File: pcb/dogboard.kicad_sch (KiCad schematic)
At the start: 32 parts, among them J1 USB-C / USB2.0, SW2 BOOT, U1 RP2040, U3 4MB Flash, Y1 12 MHz

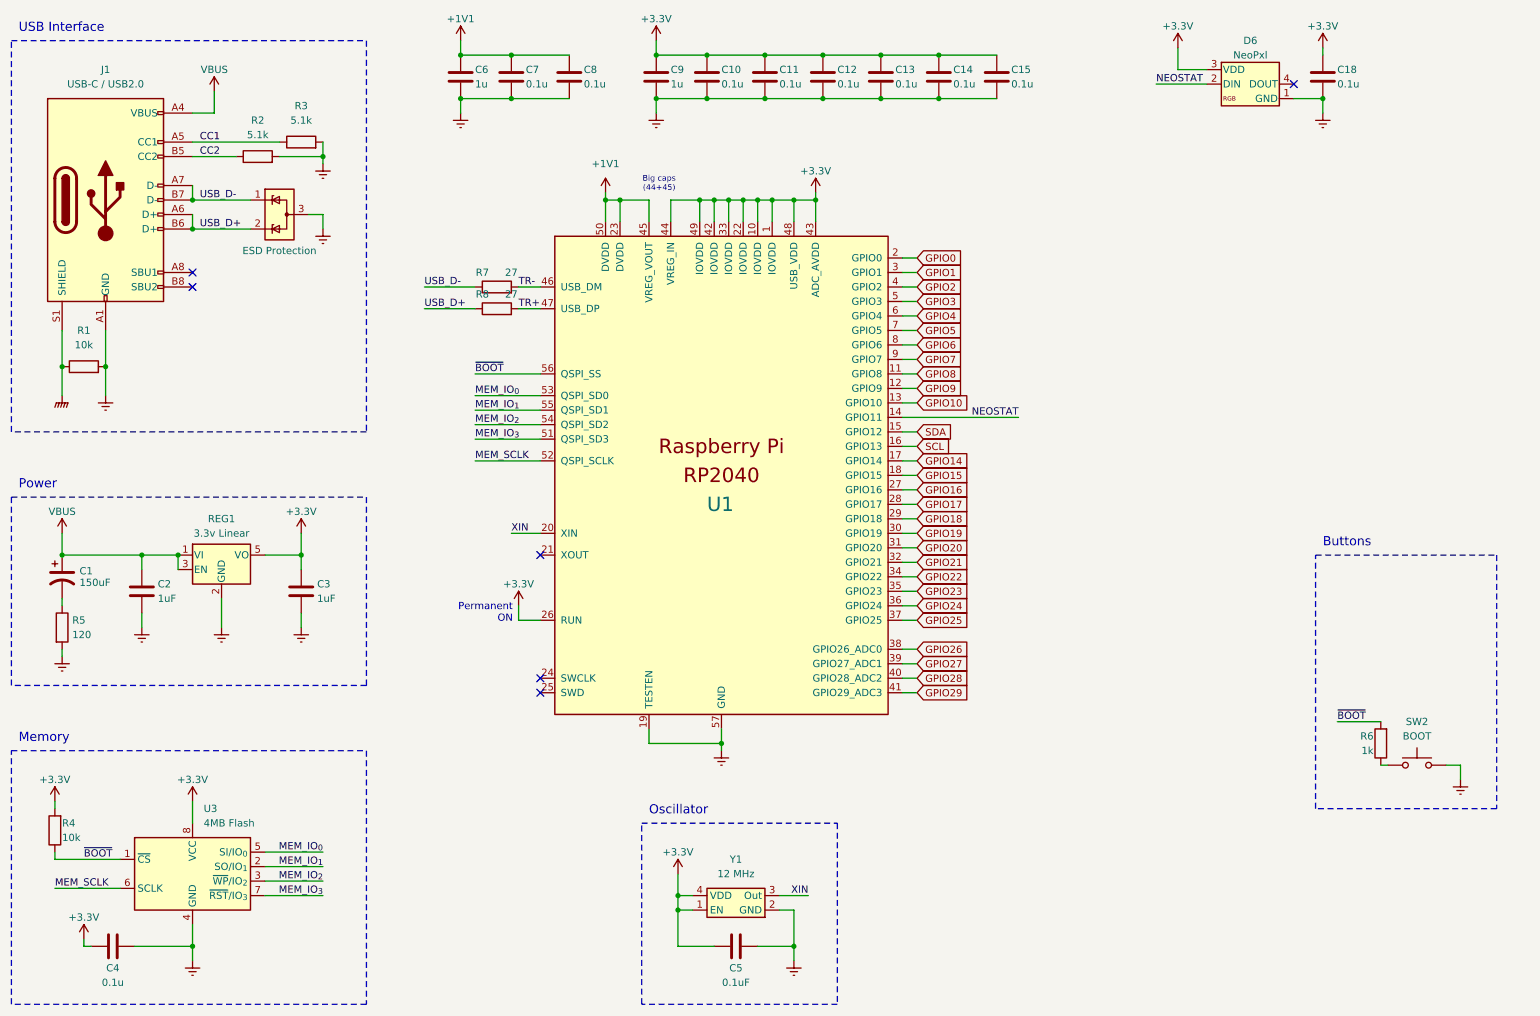
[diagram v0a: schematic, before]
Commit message: PBC rev 2 beta-1
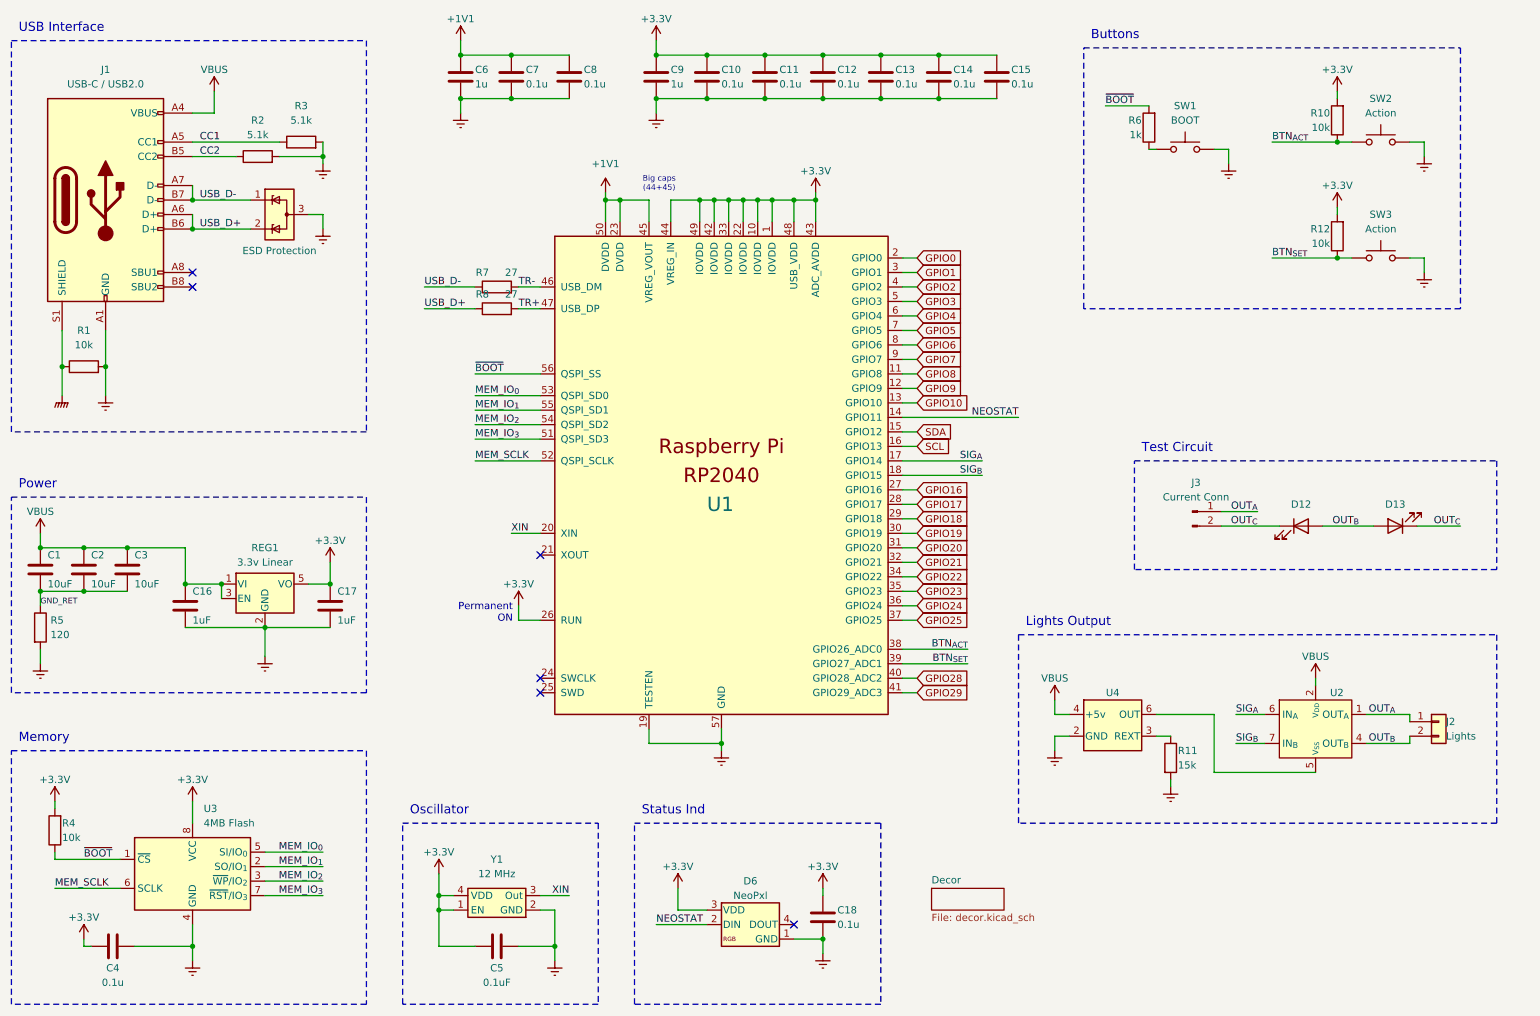
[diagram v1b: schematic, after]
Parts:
- removed C1: 150uF, _custom:CAP_Tantalum_2312, symbol _custom:CAP_Tantalum
- added C1: 10uF, _custom:CAP_1206_NoKeepout, symbol _custom:CAP_Standard
- added C16, C17: 1uF, _custom:CAP_0805_HandSolder, symbol _custom:CAP_Standard
- added D12, D13: MP-LED, _custom:LED_MP-Cathode_1113, symbol _custom:LED_Standard
- added J2: Lights, _custom:conn_1x02_JST_PH_P2.00mm_THT_Horizontal, symbol _custom:Conn_1x02
- added J3: Current Conn, Connector_PinHeader_2.54mm:PinHeader_1x02_P2.54mm_Vertical, symbol Connector:Conn_01x02_Pin
- added R10, R12: 10k, _custom:R_0805_HandSolder, symbol _custom:Resistor_Standard
- added R11: 15k, _custom:R_0805_HandSolder, symbol _custom:Resistor_Standard
- added SW2, SW3: Action, _custom:button_SMD_PTS810, symbol _custom:SW_Button_Push
- added U2: L9110H, _custom:GenericIC_TH-DIP-8, symbol _custom:L9110H_H-Bridge
- added U4: BCR430, _custom:BCR430_CC_LED_Driver, symbol _custom:BCR430_CC_LED_Driver
- C2, C3: value 1uF -> 10uF; footprint _custom:CAP_0805_HandSolder -> _custom:CAP_1206_NoKeepout
- renumbered SW2 to SW1
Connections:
- net +3.3V: now also C17.1, R10.2, R12.2; no longer C3.2
- net GNDREF: now also C16.2, C17.2, R11.2, SW2.2, SW3.2, U4.2 (GND); no longer C2.1, C3.1
- net VBUS: now also C2.1, C3.1, C1.1, C16.1, U2.2 (V_{DD}), U2.3 (V_{DD}), U4.4 (+5v); no longer C2.2
- net GND_RET: now reaches R5.1
- net GND_RET: now also C2.2, C3.2, C1.2
- net GPIO14 renamed SIG_{A}
- net SIG_{A}: now also U2.6 (IN_{A})
- net GPIO15 renamed SIG_{B}
- net SIG_{B}: now also U2.7 (IN_{B})
- net GPIO26 renamed BTN_{ACT}
- net BTN_{ACT}: now also R10.1, SW2.1
- net GPIO27 renamed BTN_{SET}
- net BTN_{SET}: now also R12.1, SW3.1
- new net: R11.1, U4.3 (REXT)
- new net OUT_{A}: J2.1 (Pin_1), J3.1 (Pin_1), U2.1 (OUT_{A})
- new net OUT_{B}: D12.2 (A), D13.2 (A), J2.2 (Pin_2), U2.4 (OUT_{B})
- new net OUT_{C}: D12.1 (K), D13.1 (K), J3.2 (Pin_2)
- new net V_{SS}: U2.5 (V_{SS}), U2.8 (V_{SS}), U4.6 (OUT)
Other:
- added sheet Decor (decor.kicad_sch)
- note added: "Lights Output"
- note added: "Status Ind"
- note added: "Test Circuit"
- moved on the sheet: C18, C5, D6, R5, R6, REG1, SW1, Y1

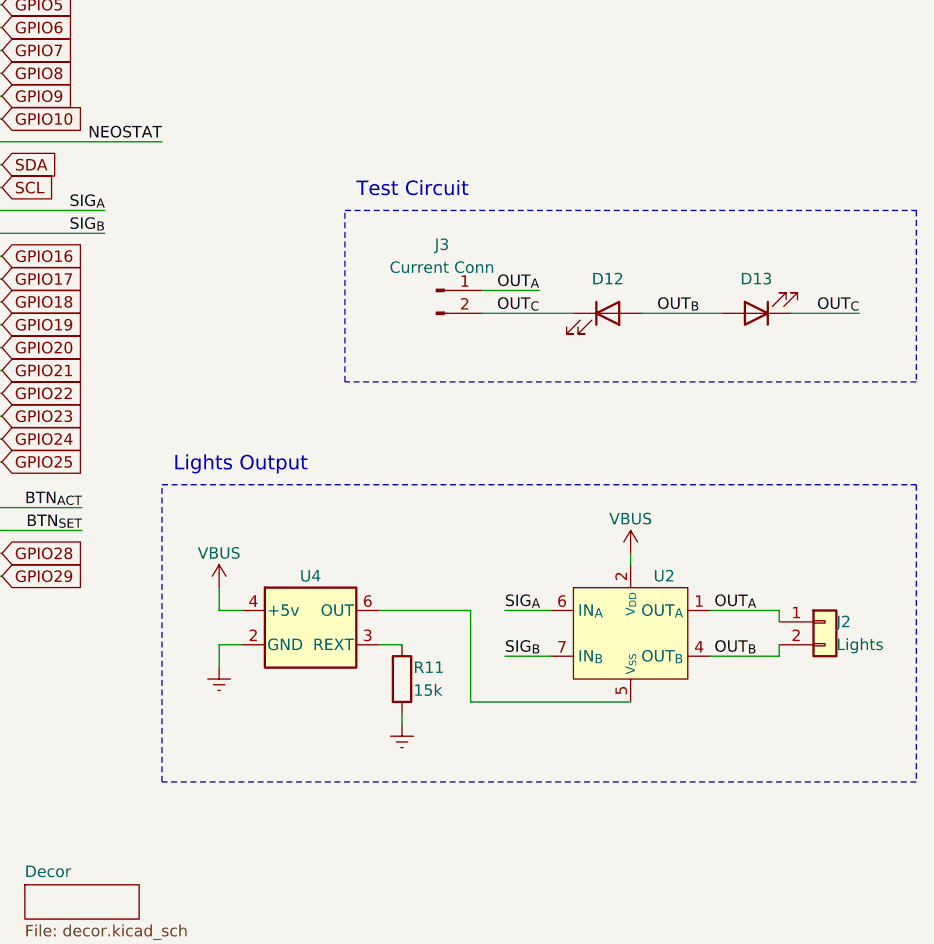
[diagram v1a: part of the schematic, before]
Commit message: PCB rev 2 beta-2
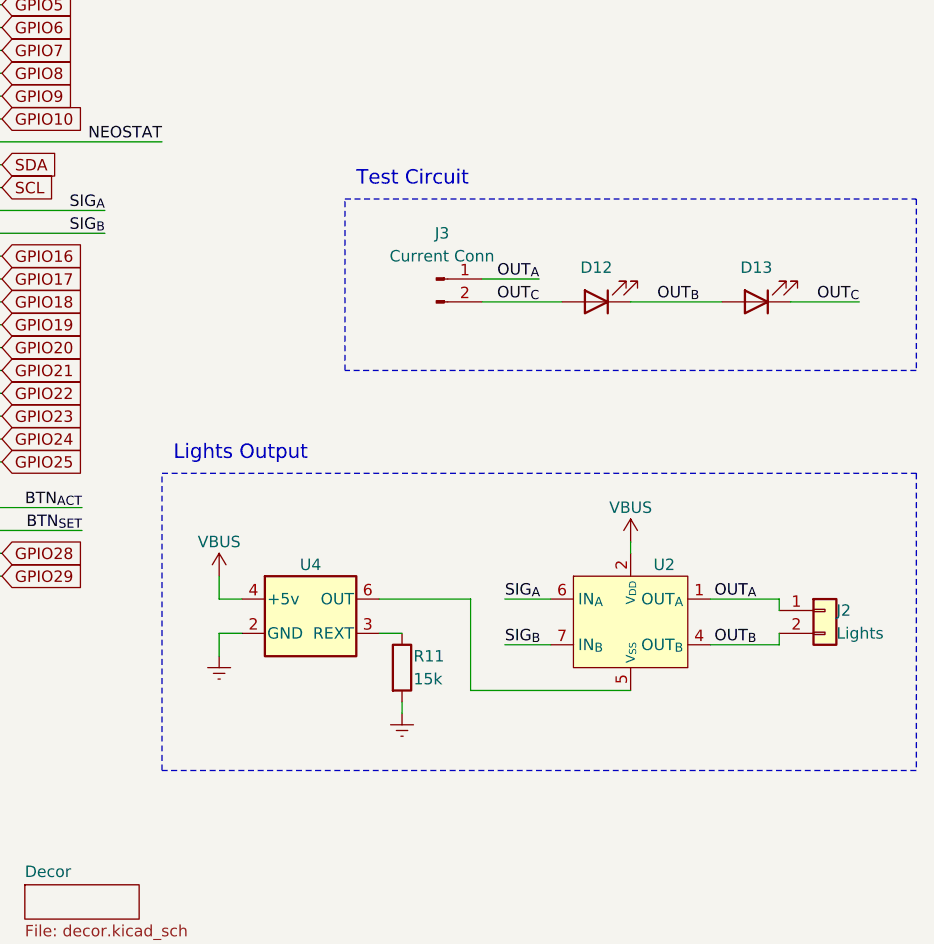
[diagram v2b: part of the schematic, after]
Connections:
- net OUT_{B}: now also D12.1 (K); no longer D12.2 (A)
- net OUT_{C}: now also D12.2 (A); no longer D12.1 (K)
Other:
- moved on the sheet: D12, D13, J2, J3, R11, U2, U4

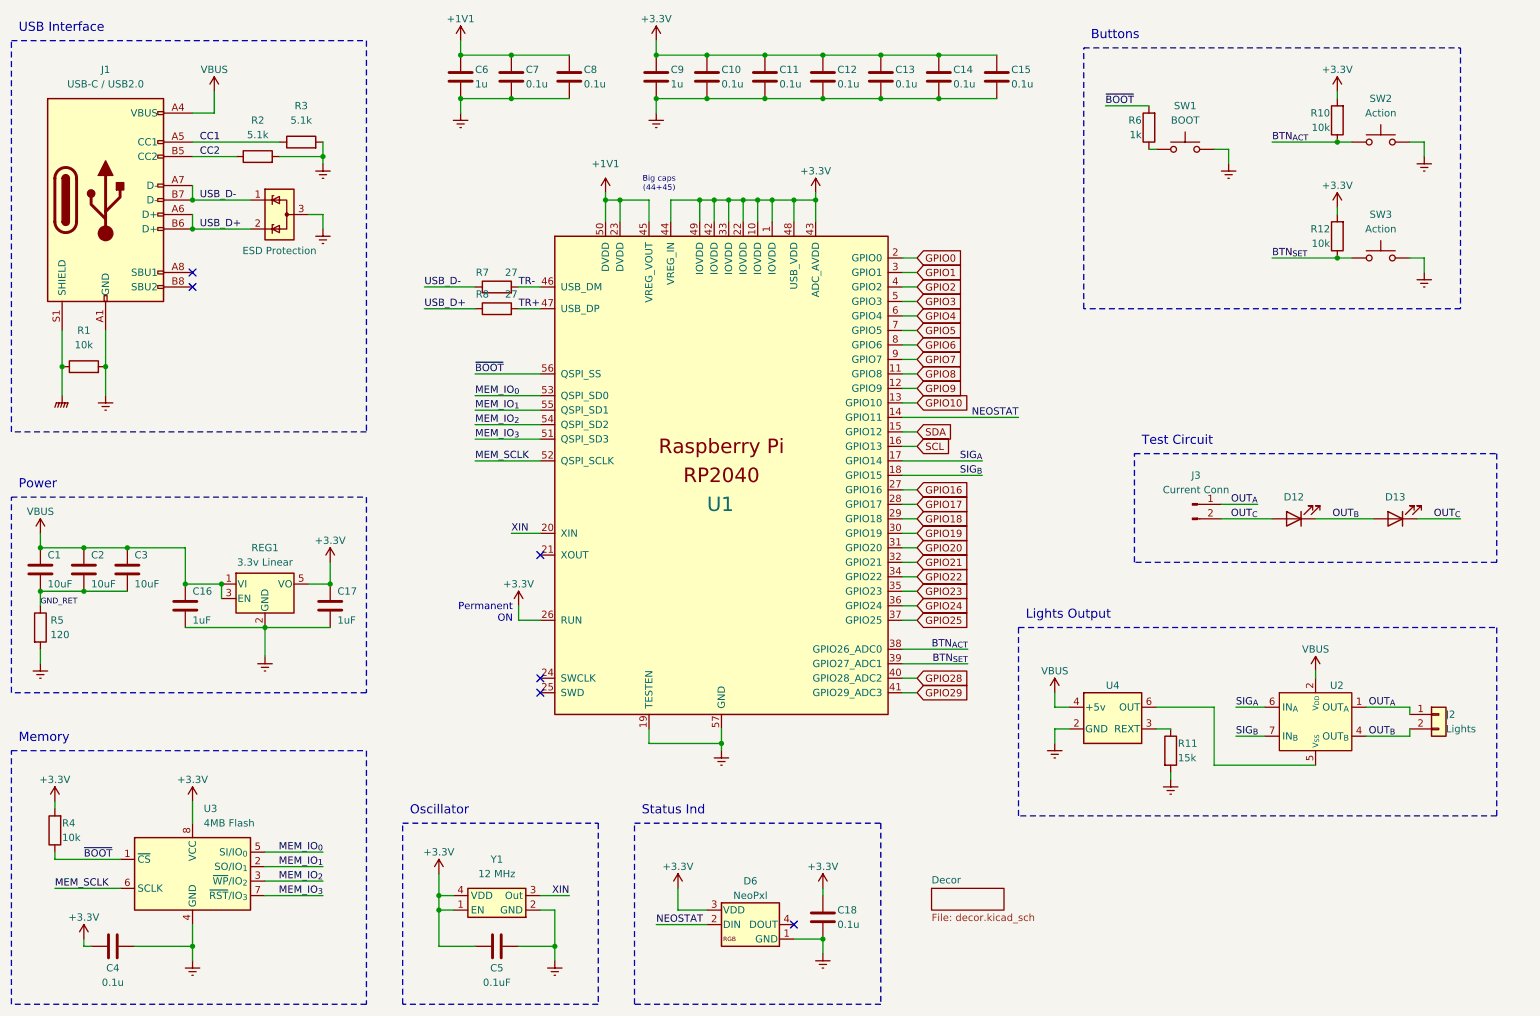
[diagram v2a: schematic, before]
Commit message: dogboard-2b3
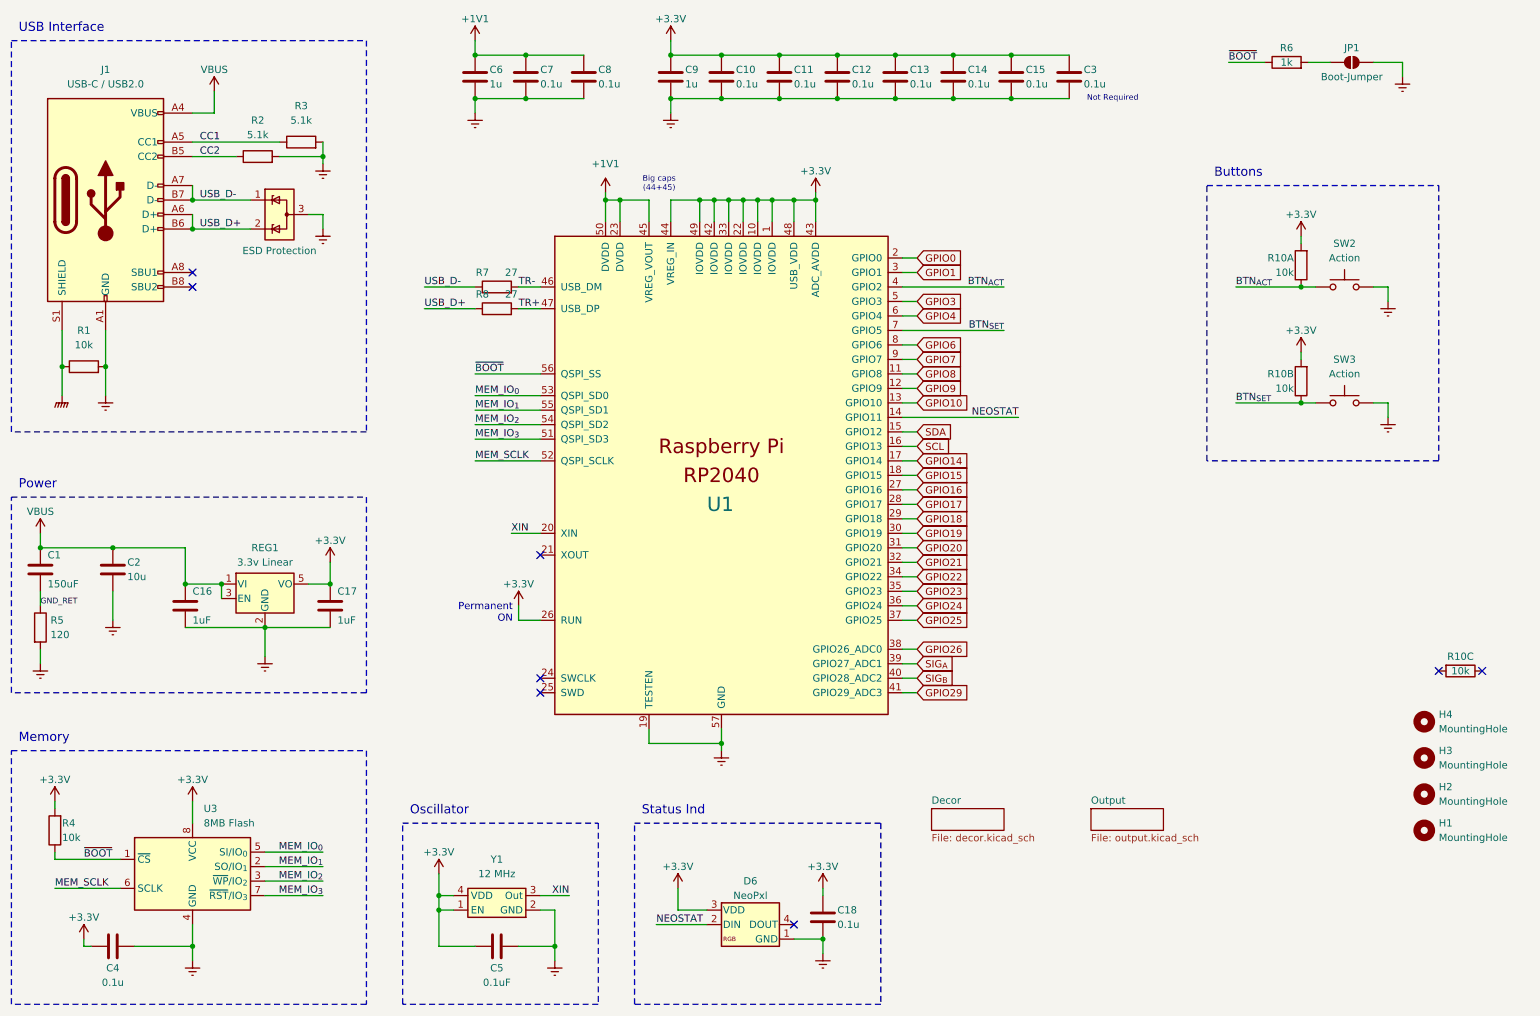
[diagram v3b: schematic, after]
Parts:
- removed D12, D13: MP-LED, _custom:LED_MP-Cathode_1113, symbol _custom:LED_Standard
- removed J2: Lights, _custom:conn_1x02_JST_PH_P2.00mm_THT_Horizontal, symbol _custom:Conn_1x02
- removed J3: Current Conn, Connector_PinHeader_2.54mm:PinHeader_1x02_P2.54mm_Vertical, symbol Connector:Conn_01x02_Pin
- removed R10, R12: 10k, _custom:R_0805_HandSolder, symbol _custom:Resistor_Standard
- removed R11: 15k, _custom:R_0805_HandSolder, symbol _custom:Resistor_Standard
- removed SW1: BOOT, _custom:button_metal_smd, symbol _custom:SW_Button_Push
- removed U2: L9110H, _custom:GenericIC_TH-DIP-8, symbol _custom:L9110H_H-Bridge
- removed U4: BCR430, _custom:BCR430_CC_LED_Driver, symbol _custom:BCR430_CC_LED_Driver
- added H1, H2, H3, H4: MountingHole, _custom:MountingHole_M2.5, symbol _custom:MountingHole
- added JP1: Boot-Jumper, _custom:Jumper_Open_SMD_3.5mm, symbol _custom:Jumper_Open
- added R10: 10k, _custom:R_Array_4x1206_Convex, symbol _custom:Resistor_Array_4x
- C1: value 10uF -> 150uF; footprint _custom:CAP_1206_NoKeepout -> _custom:CAP_Tantalum_2312
- C2: value 10uF -> 10u
- C3: value 10uF -> 0.1u; footprint _custom:CAP_1206_NoKeepout -> _custom:CAP_0402_HandSolder
- R4, R6: footprint _custom:R_0805_HandSolder -> _custom:R_0603_HandSolder
- U3: value 4MB Flash -> 8MB Flash
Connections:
- net GPIO2 is gone; now on net BTN_{ACT}: U1.4 (GPIO2)
- net GPIO28 is gone; now on net SIG_{B}: U1.40 (GPIO28_ADC2)
- net GPIO5 is gone; now on net BTN_{SET}: U1.7 (GPIO5)
- net +3.3V: now also C3.1, R10.2, R10.4
- net BTN_{ACT}: now also R10.1; no longer U1.38 (GPIO26_ADC0)
- net BTN_{SET}: now also R10.3; no longer U1.39 (GPIO27_ADC1)
- net GNDREF: now also C2.2, C3.2, JP1.2 (B)
- net GND_RET: no longer C2.2, C3.2
- net SIG_{A}: now also U1.39 (GPIO27_ADC1); no longer U1.17 (GPIO14)
- net SIG_{B}: no longer U1.18 (GPIO15)
- net VBUS: no longer C3.1
- net ~{BOOT}: now also R6.1; no longer R6.2
- new net: JP1.1 (A), R6.2
- new net GPIO14: U1.17 (GPIO14)
- new net GPIO15: U1.18 (GPIO15)
- new net GPIO26: U1.38 (GPIO26_ADC0)
- no-connect marks 6 -> 8
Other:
- added sheet Output (output.kicad_sch)
- note added: "Not Required"
- note removed: "Lights Output"
- note removed: "Test Circuit"
- moved on the sheet: C10, C11, C12, C13, C14, C15, C6, C7, C8, C9, SW2, SW3
